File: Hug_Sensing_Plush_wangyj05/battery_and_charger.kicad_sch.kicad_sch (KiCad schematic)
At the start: 16 parts, among them J2 Header B2B-PH-SM4-TBLFSN, J5 Thermistor Header TS, J6 Thermistor Header GND, U1 BQ24040DSQR

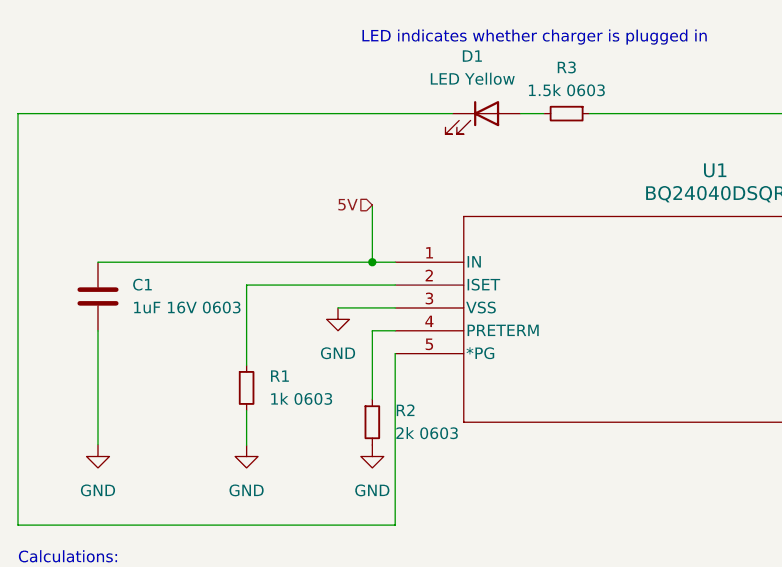
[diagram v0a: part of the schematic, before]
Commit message: Updated board layout
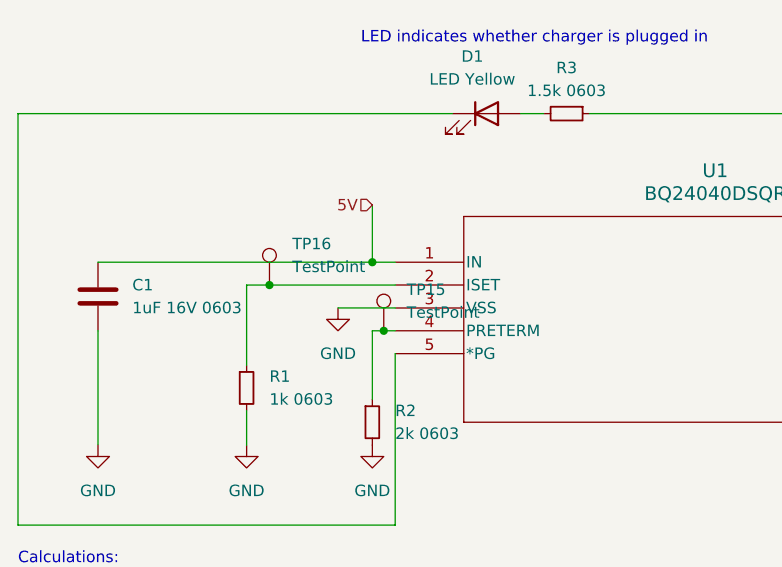
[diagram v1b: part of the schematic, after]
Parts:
- added TP15, TP16: TestPoint, TestPoint:TestPoint_Keystone_5015_Micro-Minature, symbol Connector:TestPoint
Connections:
- net at R1.1, U1.2 (ISET): now also TP16.1
- net at R2.1, U1.4 (PRETERM): now also TP15.1
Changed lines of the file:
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@@
   (junction (at 162.56 31.75) (diameter 0) (color 0 0 0 0)
   )
+  (junction (at 46.99 50.8) (diameter 0) (color 0 0 0 0)
+  )
   (junction (at 148.59 31.75) (diameter 0) (color 0 0 0 0)
+  )
+  (junction (at 59.69 55.88) (diameter 0) (color 0 0 0 0)
   )
   (junction (at 128.27 31.75) (diameter 0) (color 0 0 0 0)
@@
     (stroke (width 0) (type default))
   )
+  (wire (pts (xy 59.69 55.88) (xy 60.96 55.88))
+    (stroke (width 0) (type default))
+  )
   (wire (pts (xy 143.51 31.75) (xy 148.59 31.75))
     (stroke (width 0) (type default))
@@
     (stroke (width 0) (type default))
   )
+  (wire (pts (xy 46.99 50.8) (xy 60.96 50.8))
+    (stroke (width 0) (type default))
+  )
   (wire (pts (xy 44.45 64.77) (xy 44.45 68.58))
     (stroke (width 0) (type default))
@@
     (stroke (width 0) (type default))
   )
-  (wire (pts (xy 58.42 55.88) (xy 60.96 55.88))
+  (wire (pts (xy 58.42 55.88) (xy 59.69 55.88))
     (stroke (width 0) (type default))
   )
@@
     (stroke (width 0) (type default))
   )
-  (wire (pts (xy 44.45 50.8) (xy 60.96 50.8))
+  (wire (pts (xy 44.45 50.8) (xy 46.99 50.8))
     (stroke (width 0) (type default))
   )
@@
     )
   )
+  (symbol (lib_id "Connector:TestPoint") (at 59.69 55.88 0) (unit 1)
+    (in_bom yes) (on_board yes) (dnp no) (fields_autoplaced)
+    (property "Reference" "TP15" (at 62.23 51.308 0)
+      (effects (font (size 1.27 1.27)) (justify left))
+    )
+    (property "Value" "TestPoint" (at 62.23 53.848 0)
+      (effects (font (size 1.27 1.27)) (justify left))
+    )
+    (property "Footprint" "TestPoint:TestPoint_Keystone_5015_Micro-Minature" (at 64.77 55.88 0)
+      (effects (font (size 1.27 1.27)) hide)
+    )
+    (property "Datasheet" "https://www.koaspeer.com/pdfs/RC.pdf" (at 64.77 55.88 0)
+      (effects (font (size 1.27 1.27)) hide)
+    )
+    (property "Digikey PN" "2019-RCWCTECT-ND" (at 59.69 55.88 0)
+      (effects (font (size 1.27 1.27)) hide)
+    )
+    (property "MPN" "RCWCTE" (at 59.69 55.88 0)
+      (effects (font (size 1.27 1.27)) hide)
+    )
+    (pin "1")
+    (instances
+      (project "Hug_Sensing_Plush_wangyj05"
+        (path "/352d7abe-fc72-4473-8b68-62eecf44f496/fe114d8a-1666-439d-b237-f63ce920121d"
+          (reference "TP15") (unit 1)
+        )
+      )
+    )
+  )
   (symbol (lib_id "Device:C") (at 162.56 41.91 0) (unit 1)
     (in_bom yes) (on_board yes) (dnp no)
@@
         )
       )
+    )
+  )
+  (symbol (lib_id "Connector:TestPoint") (at 46.99 50.8 0) (unit 1)
+    (in_bom yes) (on_board yes) (dnp no) (fields_autoplaced)
+    (property "Reference" "TP16" (at 49.53 46.228 0)
+      (effects (font (size 1.27 1.27)) (justify left))
+    )
+    (property "Value" "TestPoint" (at 49.53 48.768 0)
+      (effects (font (size 1.27 1.27)) (justify left))
+    )
+    (property "Footprint" "TestPoint:TestPoint_Keystone_5015_Micro-Minature" (at 52.07 50.8 0)
+      (effects (font (size 1.27 1.27)) hide)
+    )
+    (property "Datasheet" "https://www.koaspeer.com/pdfs/RC.pdf" (at 52.07 50.8 0)
+      (effects (font (size 1.27 1.27)) hide)
+    )
+    (property "Digikey PN" "2019-RCWCTECT-ND" (at 46.99 50.8 0)
+      (effects (font (size 1.27 1.27)) hide)
+    )
+    (property "MPN" "RCWCTE" (at 46.99 50.8 0)
+      (effects (font (size 1.27 1.27)) hide)
+    )
+    (pin "1")
+    (instances
+      (project "Hug_Sensing_Plush_wangyj05"
+        (path "/352d7abe-fc72-4473-8b68-62eecf44f496/fe114d8a-1666-439d-b237-f63ce920121d"
+          (reference "TP16") (unit 1)
+        )
+      )
